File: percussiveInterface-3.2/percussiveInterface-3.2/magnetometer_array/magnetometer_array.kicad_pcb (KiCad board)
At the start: 4 copper layers, 122.6 x 14 mm, 33 parts, among them J2 Conn_01x21_Pin, U1 SM225-10E, U10 SM225-10E, U11 SM225-10E, U12 SM225-10E, U13 SM225-10E, U14 SM225-10E, U15 SM225-10E, U16 SM225-10E, U2 SM225-10E, U3 SM225-10E, U4 SM225-10E, U5 SM225-10E, U6 SM225-10E, U7 SM225-10E, U8 SM225-10E, U9 SM225-10E

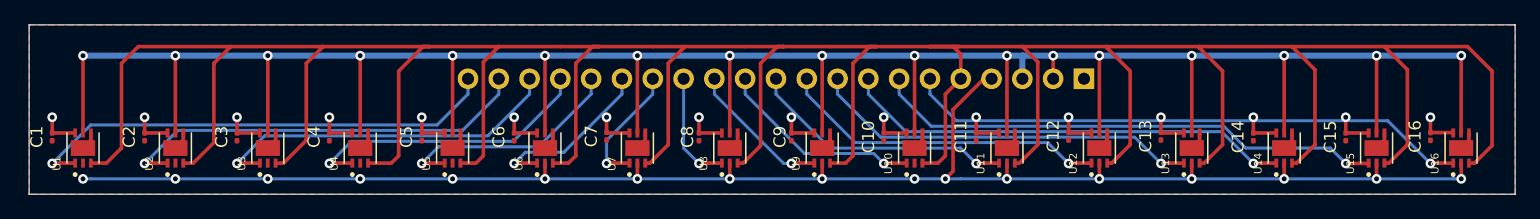
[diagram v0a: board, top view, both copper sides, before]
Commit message: stuff
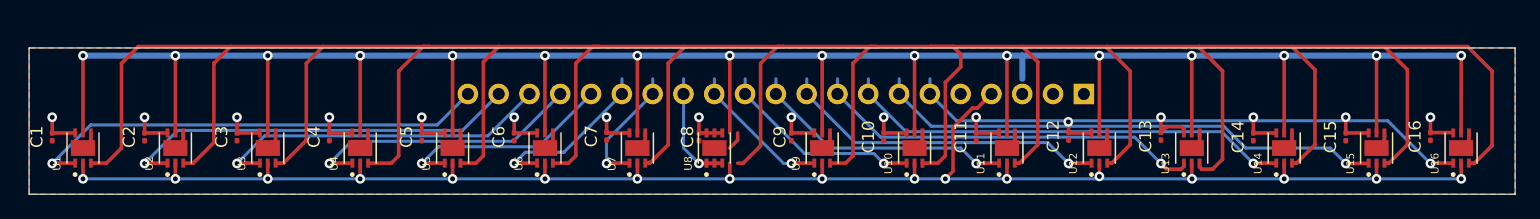
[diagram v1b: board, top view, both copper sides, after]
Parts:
- J2: footprint Connector_PinHeader_2.54mm:PinHeader_1x21_P2.54mm_Horizontal -> Connector_PinHeader_2.54mm:PinHeader_1x21_P2.54mm_Vertical
- moved U8 1.27 mm to (156.2, 111.8)
- moved J2 1.26 mm to (186.7, 107.3)
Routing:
- net MOSI: track 136.8 -> 143.0 mm
- net v+: track 52.7 -> 51.1 mm, vias 17 -> 16
- net SS5: track 19.5 -> 18.2 mm
- net SS4: track 24.6 -> 23.3 mm
- net SS3: track 29.7 -> 28.4 mm
- net SS2: track 34.7 -> 33.5 mm
- net SS1: track 39.8 -> 38.6 mm
- net MISO: track 299.7 -> 300.5 mm
- net SS13: track 32.2 -> 32.8 mm
- added copper zone on In2.Cu, net GND
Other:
- board size 122.6 x 14 mm -> 122.6 x 12.1 mm
